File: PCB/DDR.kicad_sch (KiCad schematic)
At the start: 65 parts, among them U4 STM32MP157FABx, U5 MT41K256M16TW-107_P

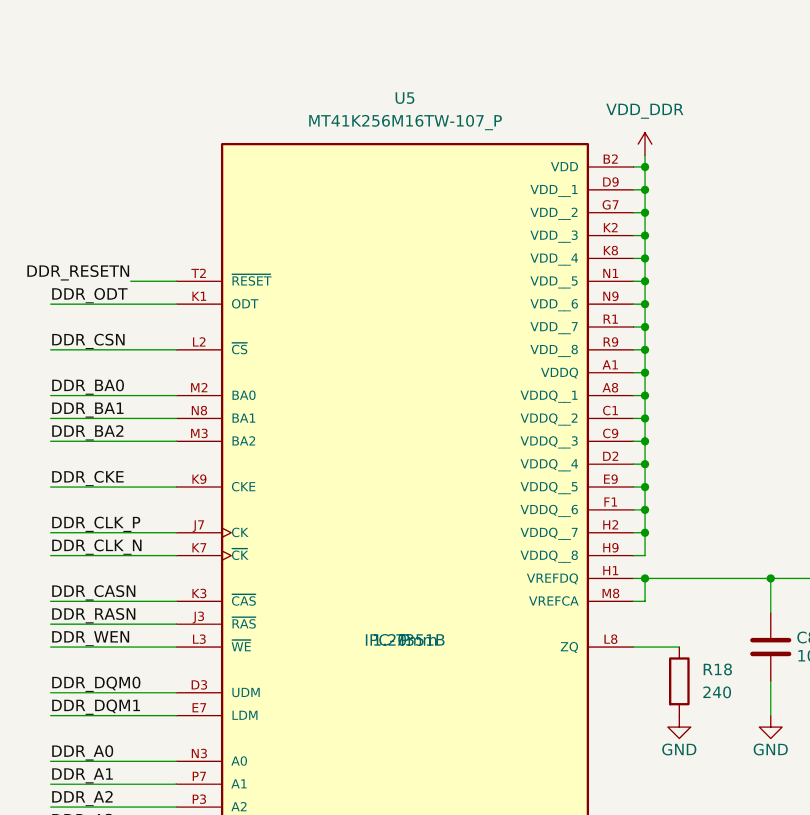
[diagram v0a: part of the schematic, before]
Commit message: update
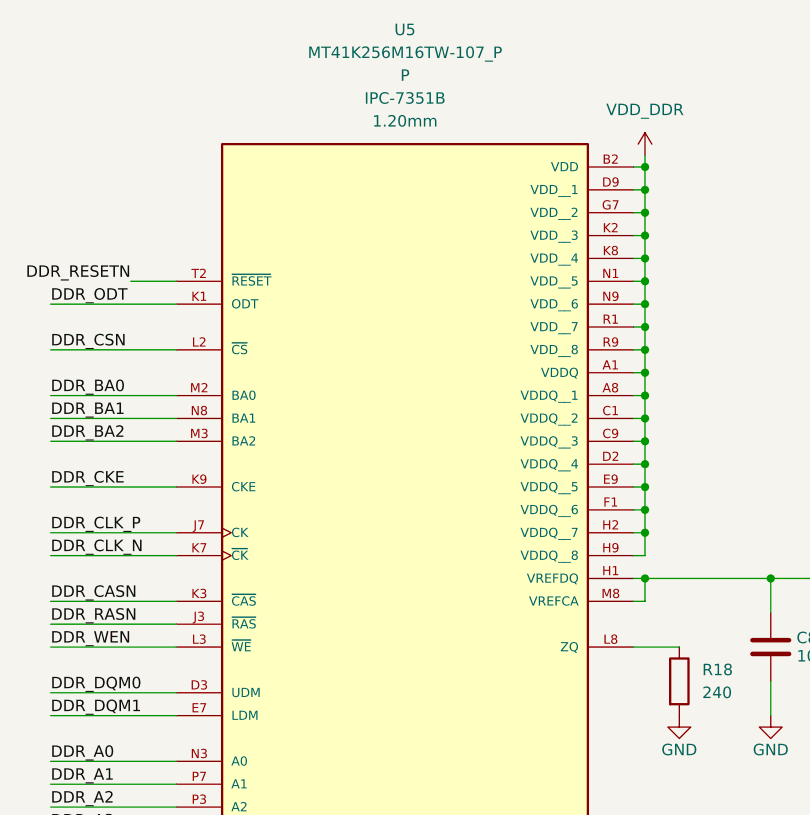
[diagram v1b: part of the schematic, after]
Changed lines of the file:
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@@
 		(fields_autoplaced yes)
 		(property "Reference" "U5"
-			(at 241.3 20.32 0)
+			(at 241.3 12.7 0)
 			(effects
 				(font
@@
 		)
 		(property "Value" "MT41K256M16TW-107_P"
-			(at 241.3 22.86 0)
+			(at 241.3 15.24 0)
 			(effects
 				(font
@@
 		)
 		(property "PARTREV" "P"
-			(at 241.3 81.28 0)
+			(at 241.3 17.78 0)
 			(effects
 				(font
 					(size 1.27 1.27)
 				)
-				(justify bottom)
 			)
 		)
 		(property "STANDARD" "IPC-7351B"
-			(at 241.3 81.28 0)
+			(at 241.3 20.32 0)
 			(effects
 				(font
 					(size 1.27 1.27)
 				)
-				(justify bottom)
 			)
 		)
 		(property "MAXIMUM_PACKAGE_HEIGHT" "1.20mm"
-			(at 241.3 81.28 0)
+			(at 241.3 22.86 0)
 			(effects
 				(font
 					(size 1.27 1.27)
 				)
-				(justify bottom)
 			)
 		)
